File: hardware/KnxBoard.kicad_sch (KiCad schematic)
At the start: 40 parts, among them J1 Conn_01x10, J2 Conn_01x12, J3 Conn_01x12, J4 Conn_01x02_Male, U1 NCN5130, U3 STM32L432KCUx, X1 FA-238

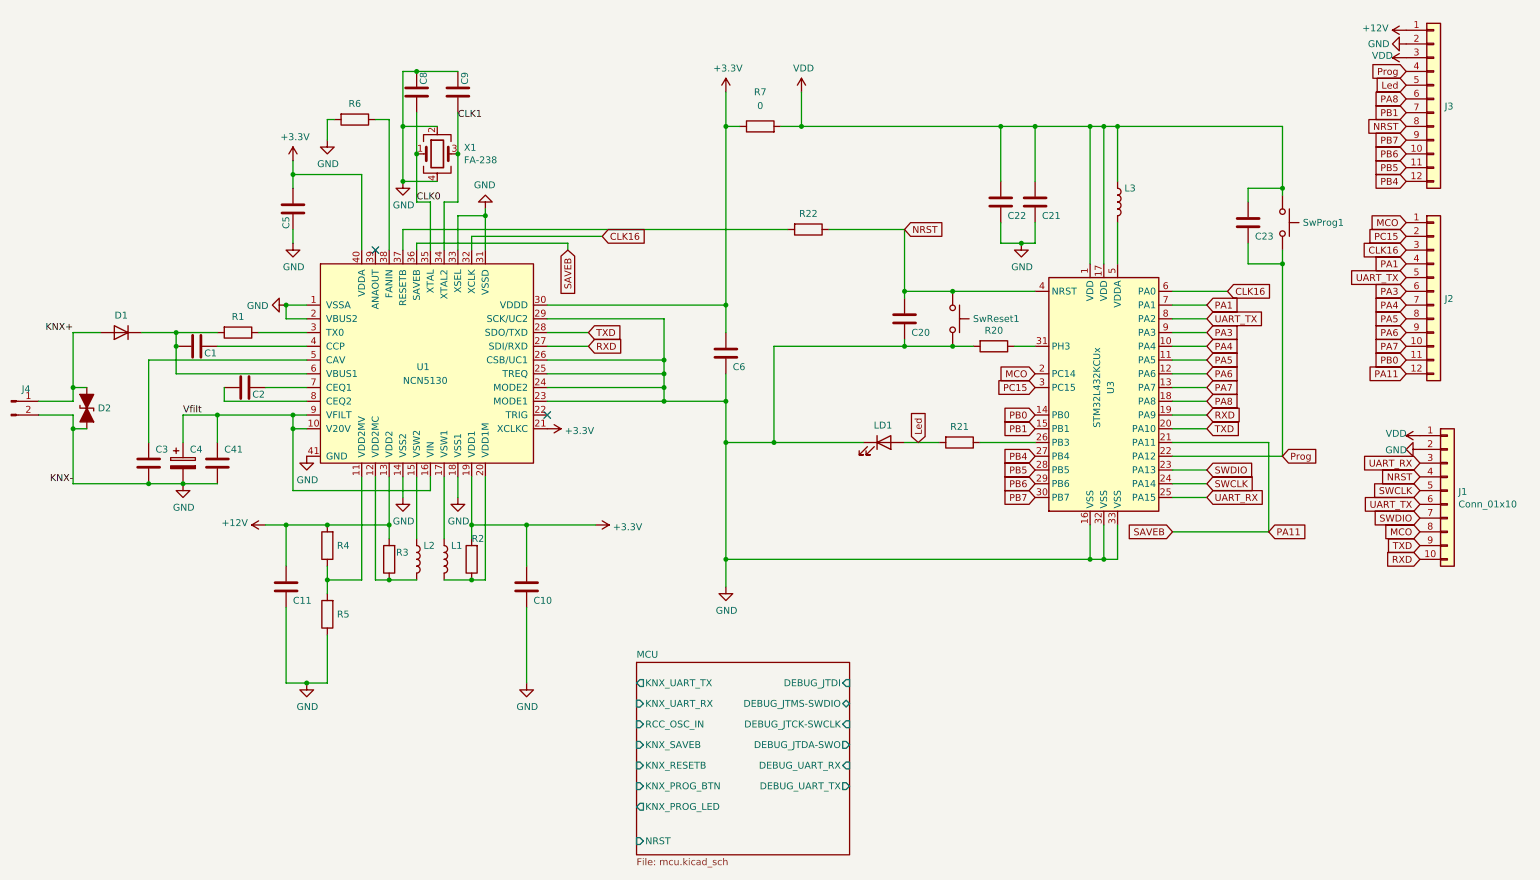
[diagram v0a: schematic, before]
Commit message: Work in progress
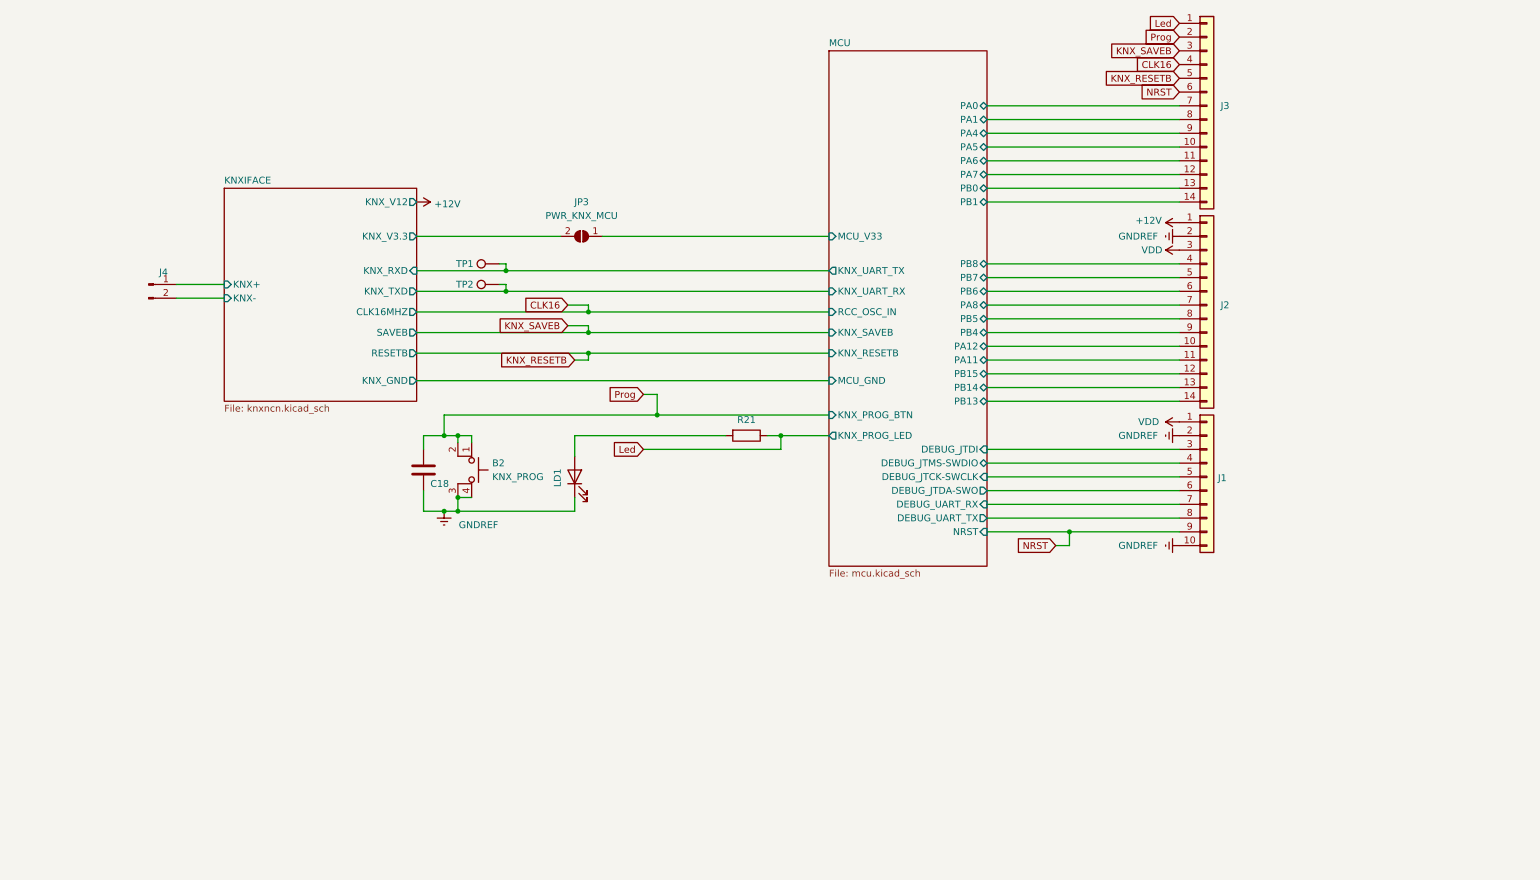
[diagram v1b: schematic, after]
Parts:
- removed C1: 47nF 50V, Capacitor_SMD:C_0603_1608Metric, symbol Device:C
- removed C10, C11, C22: 10uF 6.3V ESR < 0.1ohm, Capacitor_SMD:C_0805_2012Metric, symbol Device:C
- removed C2: 220nF 50V, Capacitor_SMD:C_0603_1608Metric, symbol Device:C
- removed C20, C21, C23, C5, C6: 100nF 6.3V, Capacitor_SMD:C_0603_1608Metric, symbol Device:C
- removed C3: 100nF 50V, Capacitor_SMD:C_0603_1608Metric, symbol Device:C
- removed C4: 100uF 35V, Capacitor_SMD:CP_Elec_6.3x7.7, symbol KnxBoard-rescue:CP-Device
- removed C41: 1uF 35V ESR < 2ohm, Capacitor_SMD:C_0603_1608Metric, symbol Device:C
- removed C8, C9: 10pF 6.3V, Capacitor_SMD:C_0603_1608Metric, symbol Device:C
- removed D1: SS16, Diode_SMD:D_SMA, symbol Device:D
- removed D2: 1SMA40CA, Diode_SMD:D_SMA, symbol KnxBoard-rescue:D_TVS_ALT-Device
- removed J2, J3: Conn_01x12, Connector_PinHeader_2.54mm:PinHeader_1x12_P2.54mm_Vertical, symbol Connector_Generic:Conn_01x12
- removed L1, L2, L3: 220uH, Inductor_SMD:L_1008_2520Metric, symbol Device:L
- removed R1: 27R 1W, Resistor_SMD:R_0612_1632Metric, symbol Device:R
- removed R2, R3: 1R 1/16W, Resistor_SMD:R_0603_1608Metric, symbol Device:R
- removed R20: 10K 1/16w, Resistor_SMD:R_0603_1608Metric, symbol Device:R
- removed R22, R6: NOTMOUNT, Resistor_SMD:R_0603_1608Metric, symbol Device:R
- removed R4: 56K 1/16w, Resistor_SMD:R_0603_1608Metric, symbol Device:R
- removed R5: 499K 1/16w, Resistor_SMD:R_0603_1608Metric, symbol Device:R
- removed R7: 0, Resistor_SMD:R_0603_1608Metric, symbol Device:R
- removed SwProg1, SwReset1: SW_Push, Button_Switch_SMD:SW_SPST_SKQG_WithStem, symbol Switch:SW_Push
- removed U1: NCN5130, Package_DFN_QFN:QFN-40-1EP_6x6mm_P0.5mm_EP4.6x4.6mm_ThermalVias, symbol KNX_NCN5130:NCN5130
- removed U3: STM32L432KCUx, Package_DFN_QFN:QFN-32-1EP_5x5mm_P0.5mm_EP3.45x3.45mm_ThermalVias, symbol MCU_ST_STM32L4:STM32L432KCUx
- removed X1: FA-238, Crystal:Crystal_SMD_SeikoEpson_FA238-4Pin_3.2x2.5mm, symbol Device:Crystal_GND24
- added B2: KNX_PROG, Button_Switch_SMD:SW_SPST_SKQG_WithStem, symbol Switch:SW_MEC_5E
- added C18: 100nF 6.3V, Capacitor_SMD:C_0603_1608Metric_Pad1.08x0.95mm_HandSolder, symbol Device:C
- added J2, J3: Conn_01x14, Connector_PinHeader_2.54mm:PinHeader_1x14_P2.54mm_Vertical, symbol Connector_Generic:Conn_01x14
- added JP3: PWR_KNX_MCU, Jumper:SolderJumper-2_P1.3mm_Open_TrianglePad1.0x1.5mm, symbol Jumper:SolderJumper_2_Open
- added TP1: KNX_RXD, TestPoint:TestPoint_Pad_D1.5mm, symbol Connector:TestPoint
- added TP2: KNX_TXD, TestPoint:TestPoint_Pad_D1.5mm, symbol Connector:TestPoint
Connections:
- net MCO is gone; now on net MCU/DEBUG_UART_TX: J1.8 (Pin_8)
- net RXD is gone; now on net GNDREF: J1.10 (Pin_10)
- net SWCLK is gone; now on net MCU/DEBUG_JTCK-SWCLK: J1.5 (Pin_5)
- net SWDIO is gone; now on net MCU/DEBUG_UART_RX: J1.7 (Pin_7)
- net TXD is gone; now on net NRST: J1.9 (Pin_9)
- net UART_RX is gone; now on net MCU/DEBUG_JTDI: J1.3 (Pin_3)
- net UART_TX is gone; now on net MCU/DEBUG_JTDA-SWO: J1.6 (Pin_6)
- net +12V: now also J2.1 (Pin_1)
- net CLK16: now also J3.4 (Pin_4)
- net Led: now also R21.1, J3.1 (Pin_1); no longer LD1.2 (A), R21.2
- net MCU/DEBUG_JTMS-SWDIO: now also J1.4 (Pin_4)
- net NRST: now also J3.6 (Pin_6); no longer J1.4 (Pin_4)
- net Prog: now also B2.1, B2.2, C18.1, J3.2 (Pin_2)
- net VDD: now also J2.3 (Pin_3)
- net GND renamed GNDREF
- net GNDREF: now also B2.3 (K), B2.4 (A), C18.2, J2.2 (Pin_2); no longer J4.2 (Pin_2)
- net KNX+ renamed KNXIFACE/KNX+
- new net: LD1.2 (A), R21.2
- new net KNXIFACE/KNX-: J4.2 (Pin_2)
- new net KNXIFACE/KNX_RXD: TP1.1
- new net KNXIFACE/KNX_TXD: TP2.1
- new net KNXIFACE/KNX_V3.3: JP3.2 (B)
- new net KNX_RESETB: J3.5 (Pin_5)
- new net KNX_SAVEB: J3.3 (Pin_3)
- new net MCU/MCU_V33: JP3.1 (A)
- new net MCU/PA0: J3.7 (Pin_7)
- new net MCU/PA1: J3.8 (Pin_8)
- new net MCU/PA11: J2.11 (Pin_11)
- new net MCU/PA12: J2.10 (Pin_10)
- new net MCU/PA4: J3.9 (Pin_9)
- new net MCU/PA5: J3.10 (Pin_10)
- new net MCU/PA6: J3.11 (Pin_11)
- new net MCU/PA7: J3.12 (Pin_12)
- new net MCU/PA8: J2.7 (Pin_7)
- new net MCU/PB0: J3.13 (Pin_13)
- new net MCU/PB1: J3.14 (Pin_14)
- new net MCU/PB13: J2.14 (Pin_14)
- new net MCU/PB14: J2.13 (Pin_13)
- new net MCU/PB15: J2.12 (Pin_12)
- new net MCU/PB4: J2.9 (Pin_9)
- new net MCU/PB5: J2.8 (Pin_8)
- new net MCU/PB6: J2.6 (Pin_6)
- new net MCU/PB7: J2.5 (Pin_5)
- new net MCU/PB8: J2.4 (Pin_4)
- no-connect marks 2 -> 0
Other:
- added sheet KNXIFACE (knxncn.kicad_sch)
- sheet MCU ports: added MCU_GND, MCU_V33, PA0, PA1, PA11, PA12, PA4, PA5, PA6, PA7, PA8, PB0, PB1, PB13, PB14, PB15, PB4, PB5, PB6, PB7, PB8; removed none
- moved on the sheet: J1, J4, LD1, R21
